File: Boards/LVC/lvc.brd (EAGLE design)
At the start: 20.3 x 20.3 mm, 21 parts, among them Q1 SI7997DP, Q2 RK7002BMT116, U1 NCP300LSN33T1G, U2 L78L33ACUTR, U3 TLV170IDBVR

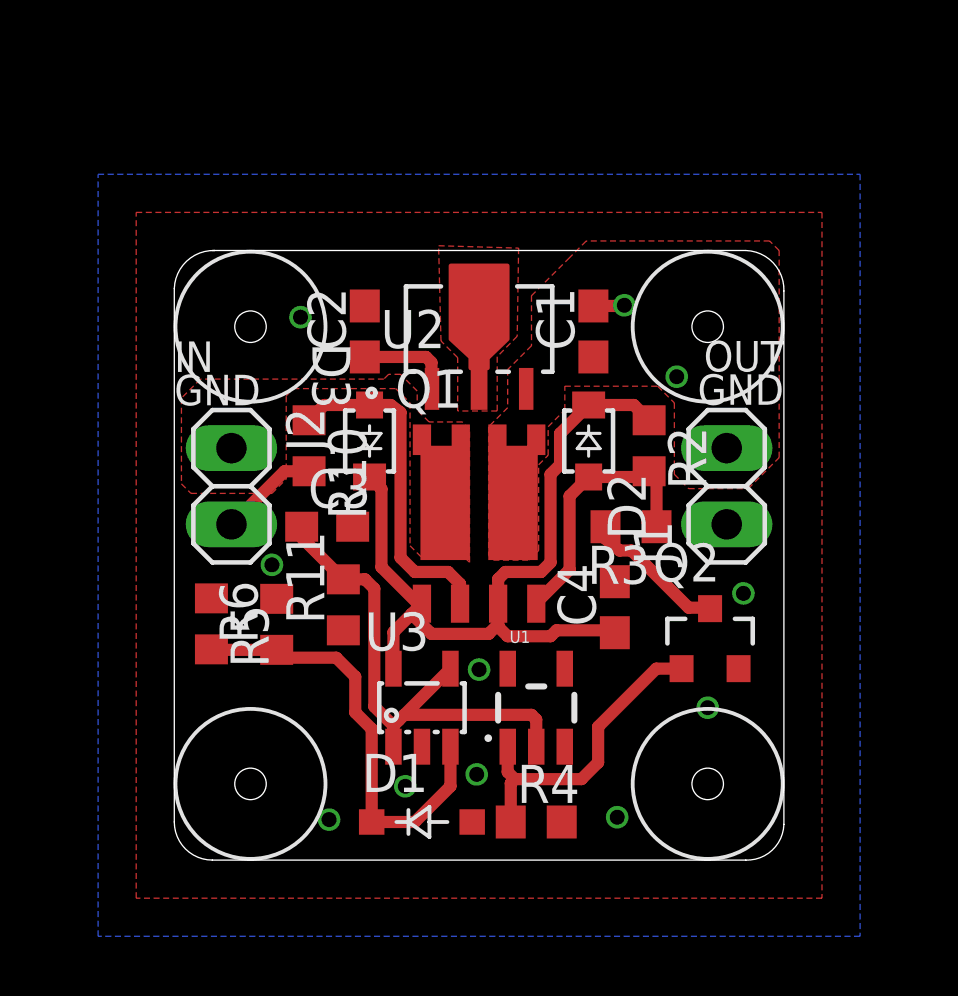
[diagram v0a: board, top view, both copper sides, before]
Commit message: a whole lot of finshed nonsense
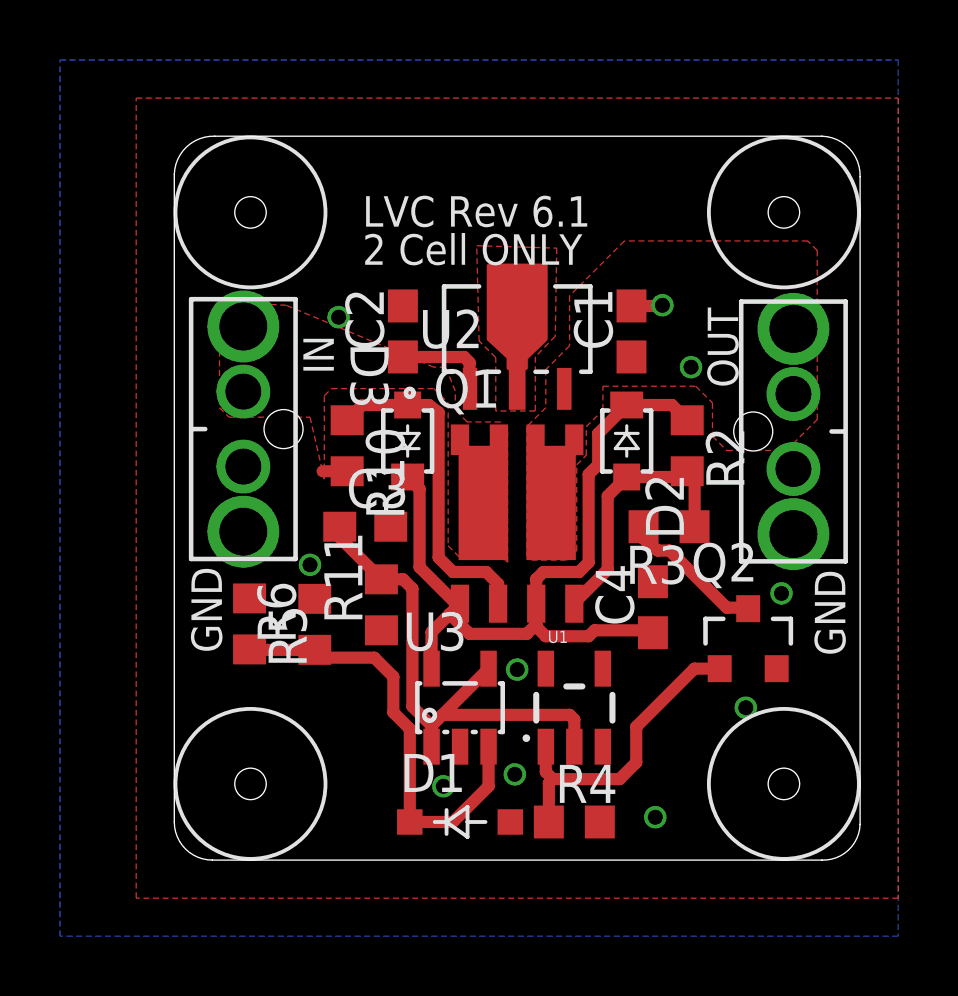
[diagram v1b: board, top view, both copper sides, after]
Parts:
- removed J1, J2: (no value), pinhead:1X02
- added U$1, U$2: MOLEX_NANOFIT_2, cmdLibs:MOLEX_NANOFIT_2
- moved C4 1.27 mm to (16.0, 8.43)
- moved D2 1.27 mm to (15.1, 14.0)
- moved R4 1.27 mm to (13.3, 1.27)
- moved U1 1.27 mm to (13.3, 5.08)
- moved C2 1.27 mm to (7.62, 17.6)
- moved R6 1.27 mm to (4.68, 7.86)
- moved R5 1.27 mm to (2.51, 7.87)
- moved C1 1.27 mm to (15.2, 17.6)
- moved C3 1.27 mm to (6.37, 11.1)
- moved D1 1.27 mm to (9.53, 1.27)
- moved D3 1.27 mm to (7.78, 14.0)
- moved Q1 1.27 mm to (11.4, 11.3)
- moved Q2 1.27 mm to (19.1, 7.38)
- moved R10 1.27 mm to (5.76, 13.8)
- moved R11 1.27 mm to (6.91, 8.51)
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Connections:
- net GND: now also U$1.P$1, U$2.P$2; no longer J1.1, J2.2
- net VDD: now also U$2.P$1; no longer J2.1
- net VOUT: now also U$1.P$2; no longer J1.2
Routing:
- net GND: track 4.36 -> 1.86 mm, vias 11 -> 10
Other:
- board size 20.3 x 20.3 mm -> 22.9 x 24.1 mm
